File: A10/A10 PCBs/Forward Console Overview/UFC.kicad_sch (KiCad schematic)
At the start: 63 parts

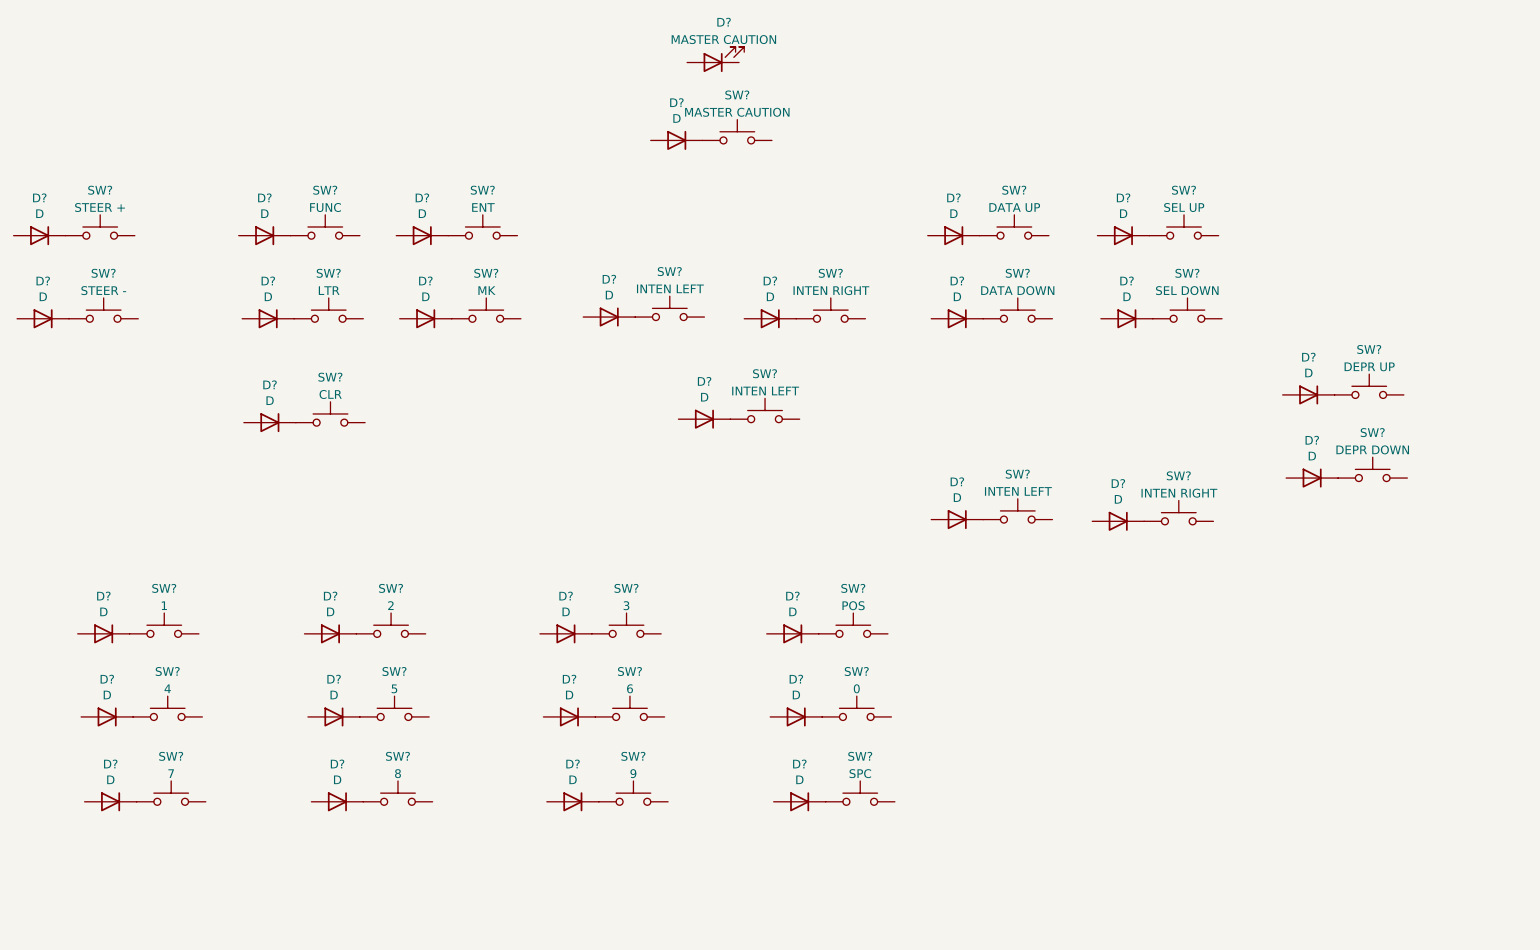
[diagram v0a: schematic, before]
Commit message: A10
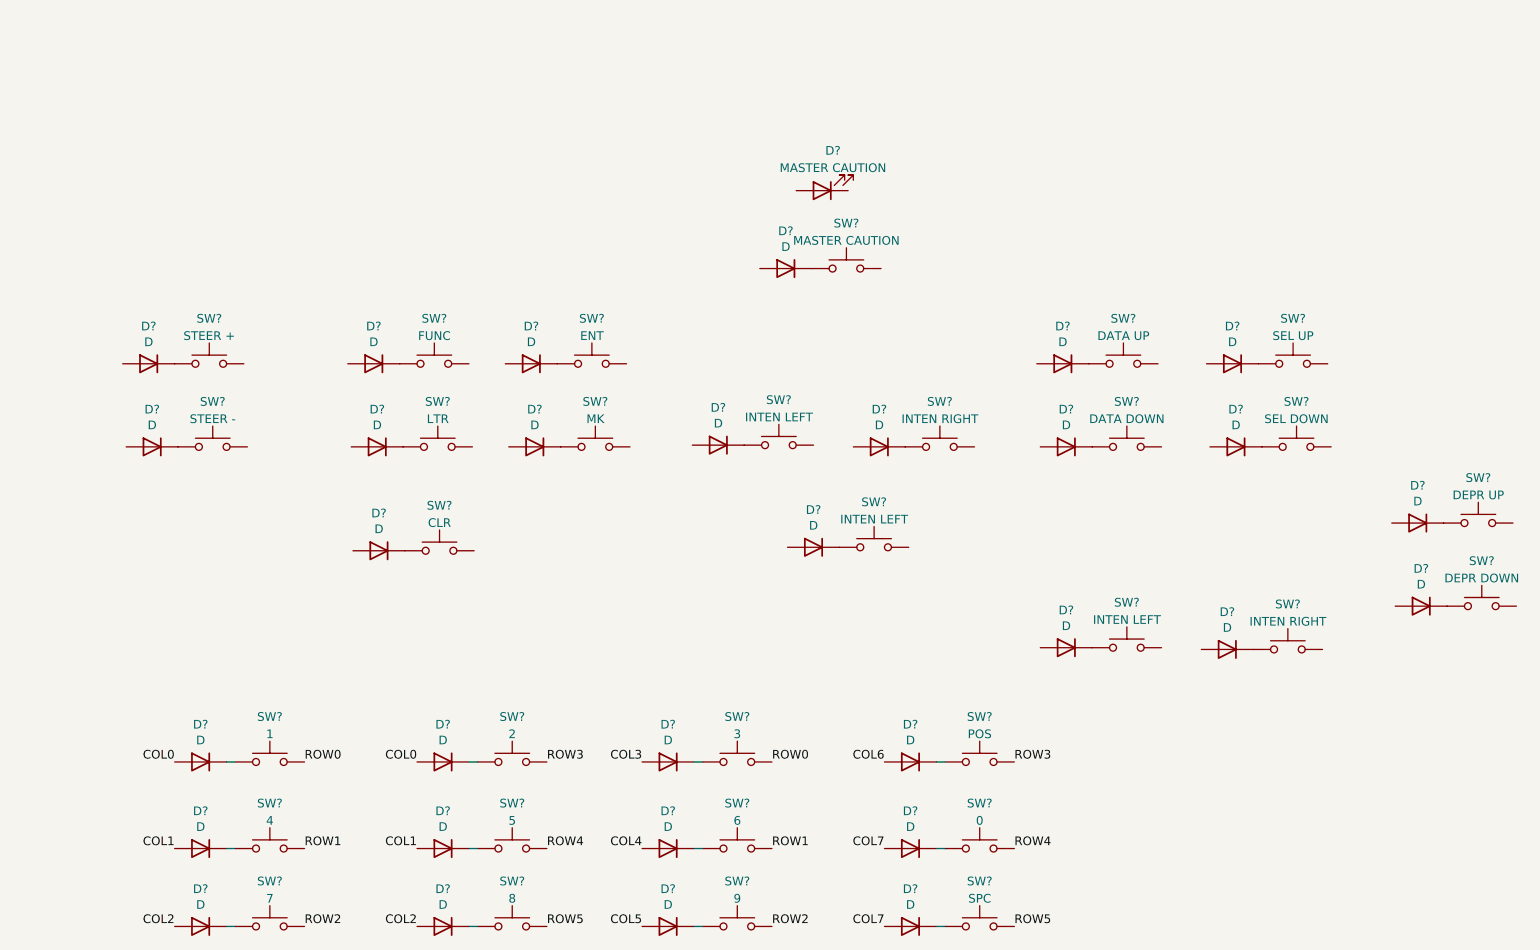
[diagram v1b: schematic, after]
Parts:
- removed D? (x6): D, Diode_THT:D_A-405_P7.62mm_Horizontal, symbol Device:D
- removed SW?: 0, Connector_Molex:Molex_KK-254_AE-6410-02A_1x02_P2.54mm_Vertical, symbol Switch:SW_Push
- removed SW?: 9, Connector_Molex:Molex_KK-254_AE-6410-02A_1x02_P2.54mm_Vertical, symbol Switch:SW_Push
- removed SW?: SPC, Connector_Molex:Molex_KK-254_AE-6410-02A_1x02_P2.54mm_Vertical, symbol Switch:SW_Push
- removed SW?: 3, Connector_Molex:Molex_KK-254_AE-6410-02A_1x02_P2.54mm_Vertical, symbol Switch:SW_Push
- removed SW?: POS, Connector_Molex:Molex_KK-254_AE-6410-02A_1x02_P2.54mm_Vertical, symbol Switch:SW_Push
- removed SW?: 6, Connector_Molex:Molex_KK-254_AE-6410-02A_1x02_P2.54mm_Vertical, symbol Switch:SW_Push
- added D? (x6): D, Diode_THT:D_A-405_P7.62mm_Horizontal, symbol Device:D
- added SW?: 6, Connector_Molex:Molex_KK-254_AE-6410-02A_1x02_P2.54mm_Vertical, symbol Switch:SW_Push
- added SW?: POS, Connector_Molex:Molex_KK-254_AE-6410-02A_1x02_P2.54mm_Vertical, symbol Switch:SW_Push
- added SW?: 9, Connector_Molex:Molex_KK-254_AE-6410-02A_1x02_P2.54mm_Vertical, symbol Switch:SW_Push
- added SW?: SPC, Connector_Molex:Molex_KK-254_AE-6410-02A_1x02_P2.54mm_Vertical, symbol Switch:SW_Push
- added SW?: 0, Connector_Molex:Molex_KK-254_AE-6410-02A_1x02_P2.54mm_Vertical, symbol Switch:SW_Push
- added SW?: 3, Connector_Molex:Molex_KK-254_AE-6410-02A_1x02_P2.54mm_Vertical, symbol Switch:SW_Push
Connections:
- net COL1: now reaches D?.2 (A)
- net COL1: now also D?.2 (A)
- net COL0: now reaches D?.2 (A)
- net COL0: now also D?.2 (A)
- net ROW5: now reaches SW?.2
- net ROW5: now also SW?.2
- net ROW0: now reaches SW?.2
- net ROW0: now also SW?.2
- net ROW4: now reaches SW?.2
- net ROW4: now also SW?.2
- net ROW1: now reaches SW?.2
- net ROW1: now also SW?.2
- net ROW2: now reaches SW?.2
- net ROW2: now also SW?.2
- net COL2: now reaches D?.2 (A)
- net COL2: now also D?.2 (A)
- net ROW3: now reaches SW?.2
- net ROW3: now also SW?.2
- new net: D?.1 (K), SW?.1 (x6)
- new net COL3: D?.2 (A)
- new net COL4: D?.2 (A)
- new net COL5: D?.2 (A)
- new net COL6: D?.2 (A)
- new net COL7: D?.2 (A), D?.2 (A)
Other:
- moved on the sheet: D?, SW?
